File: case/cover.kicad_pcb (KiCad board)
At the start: 2 copper layers, 20 x 55 mm, 5 parts

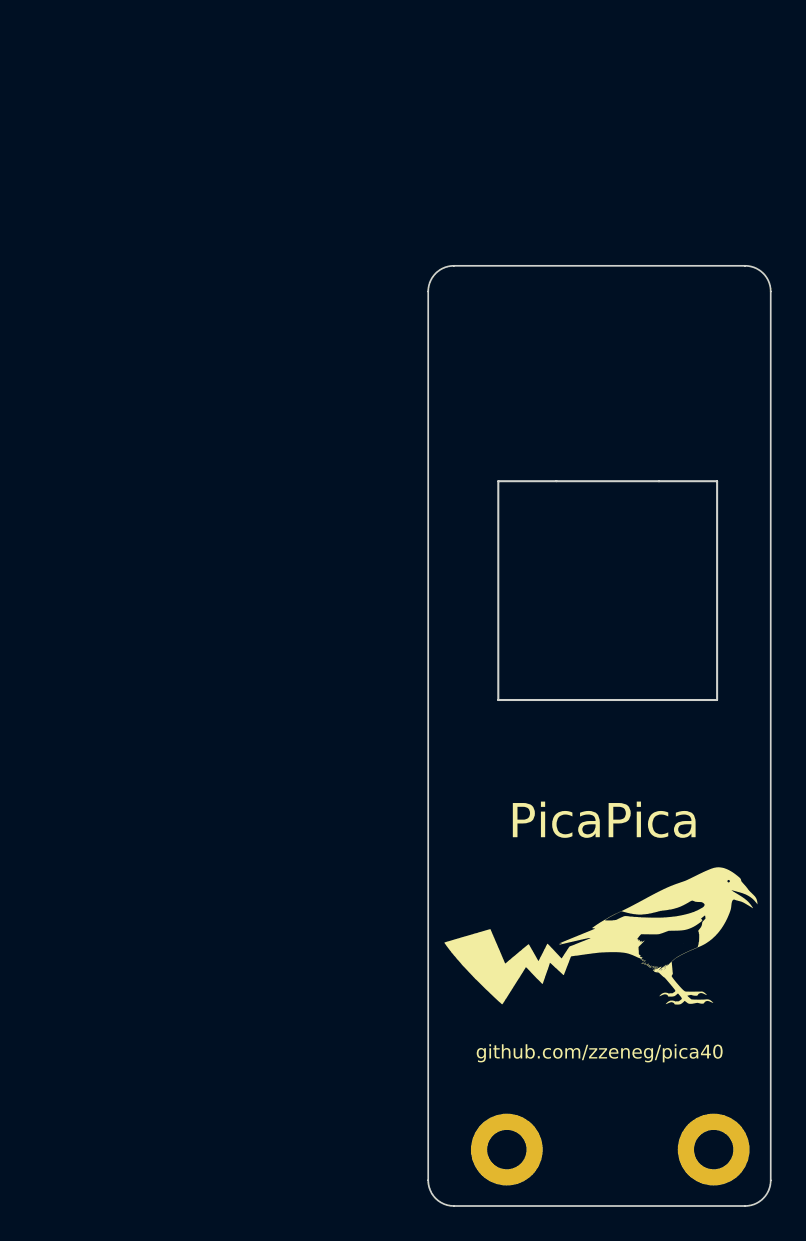
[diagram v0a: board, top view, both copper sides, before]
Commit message: update case files
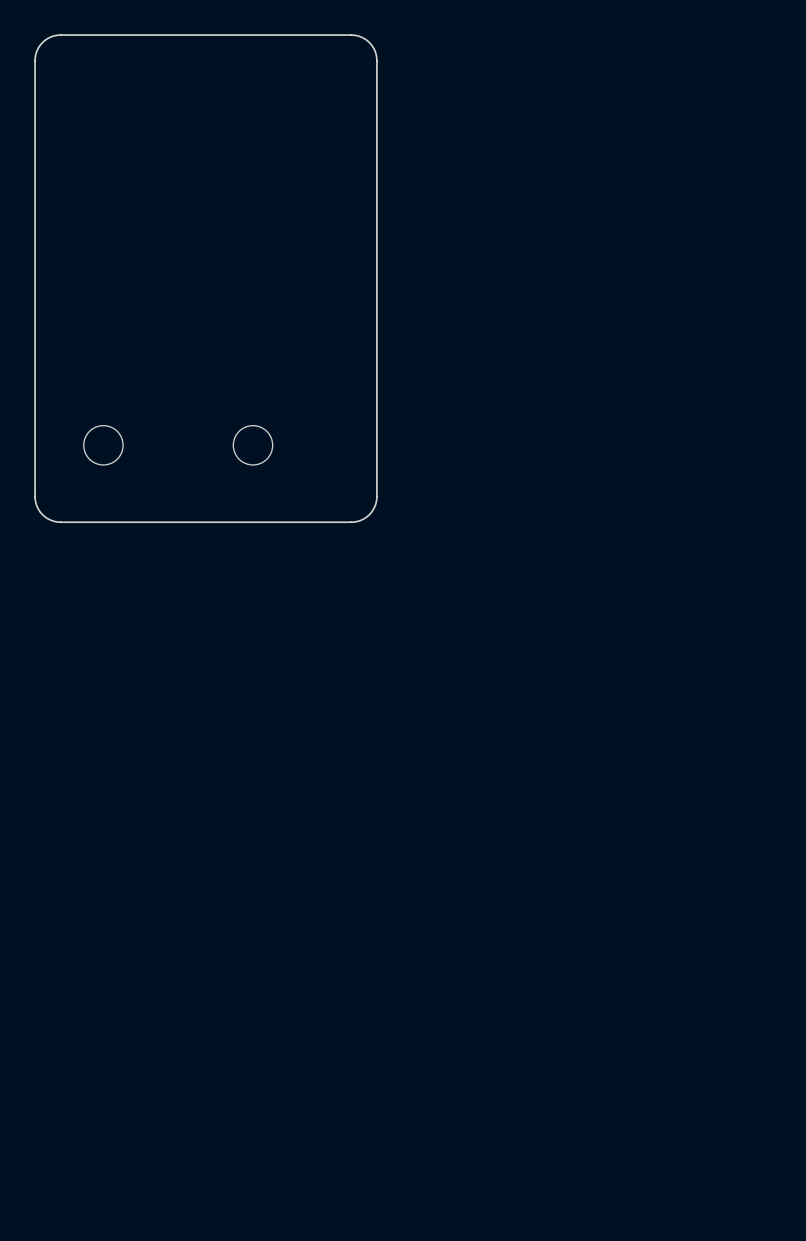
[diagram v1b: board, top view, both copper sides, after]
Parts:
- removed G***: LOGO, pica:logo_mirror
- removed G***: LOGO, pica:logo
- removed H6, H7: MountingHole, kbd:M2_Hole_TH
- removed RE1: RotaryEncoder_Switch, pica:EC11_Hole
- added Ref**: Val**, kbd:thread_m2, F.Cu at (112.8, 76.5)
- added Ref**: Val**, kbd:thread_m2, F.Cu at (104.0, 76.5)
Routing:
- net (no net): vias 1 -> 0
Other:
- board size 20 x 55 mm -> 20 x 28.5 mm
- board text removed: "JLCJLCJLCJLC"
- board text removed: "PicaPica"
- board text removed: "github.com/zzeneg/pica40"
